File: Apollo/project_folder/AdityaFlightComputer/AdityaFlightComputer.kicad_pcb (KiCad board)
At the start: 2 copper layers, 52.3 x 83.4 mm, 18 parts, among them J1 SW, J2 BAT, J3 GPS, J4 Radio, U1 LPS22HHTR, U3 LSM6DSOTR, U4 MLX90397RLQ-AAA-000-SP

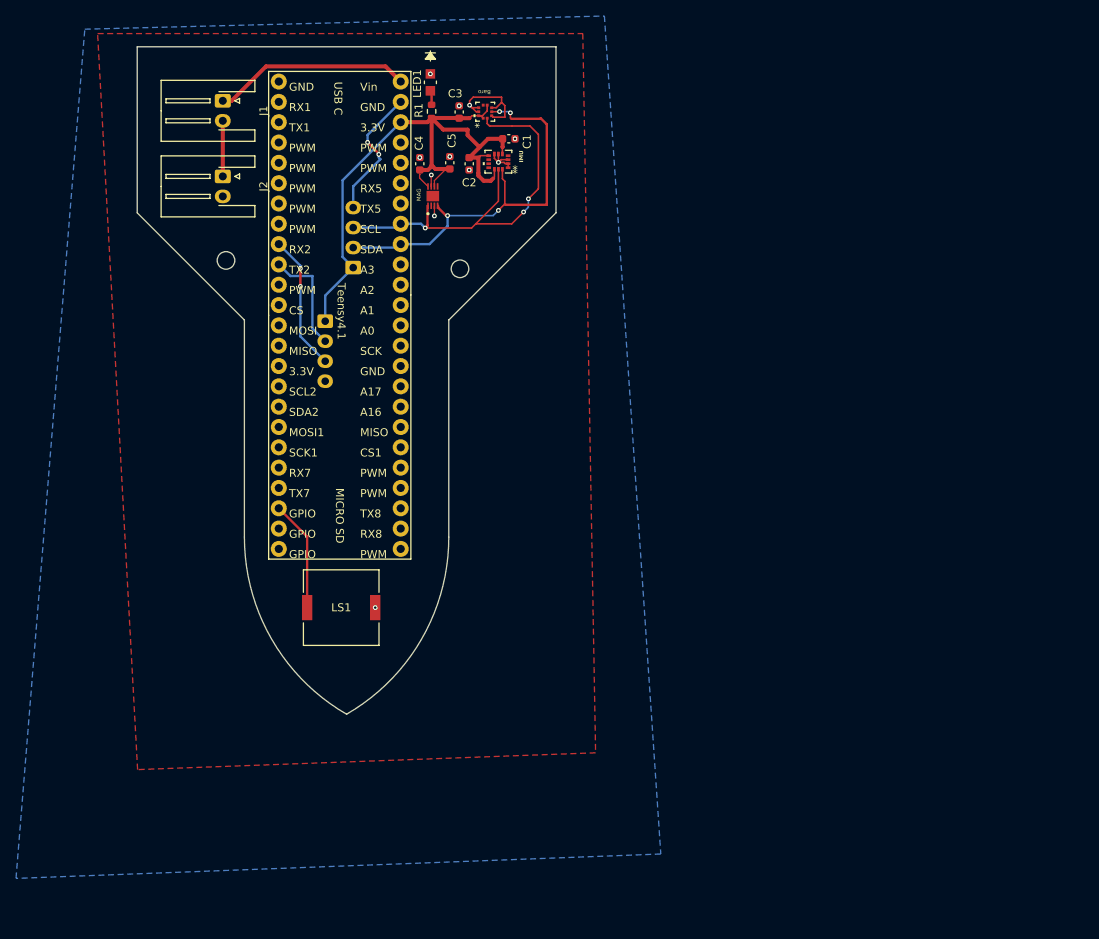
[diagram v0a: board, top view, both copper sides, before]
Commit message: autejwani
Fixed Flight Controller
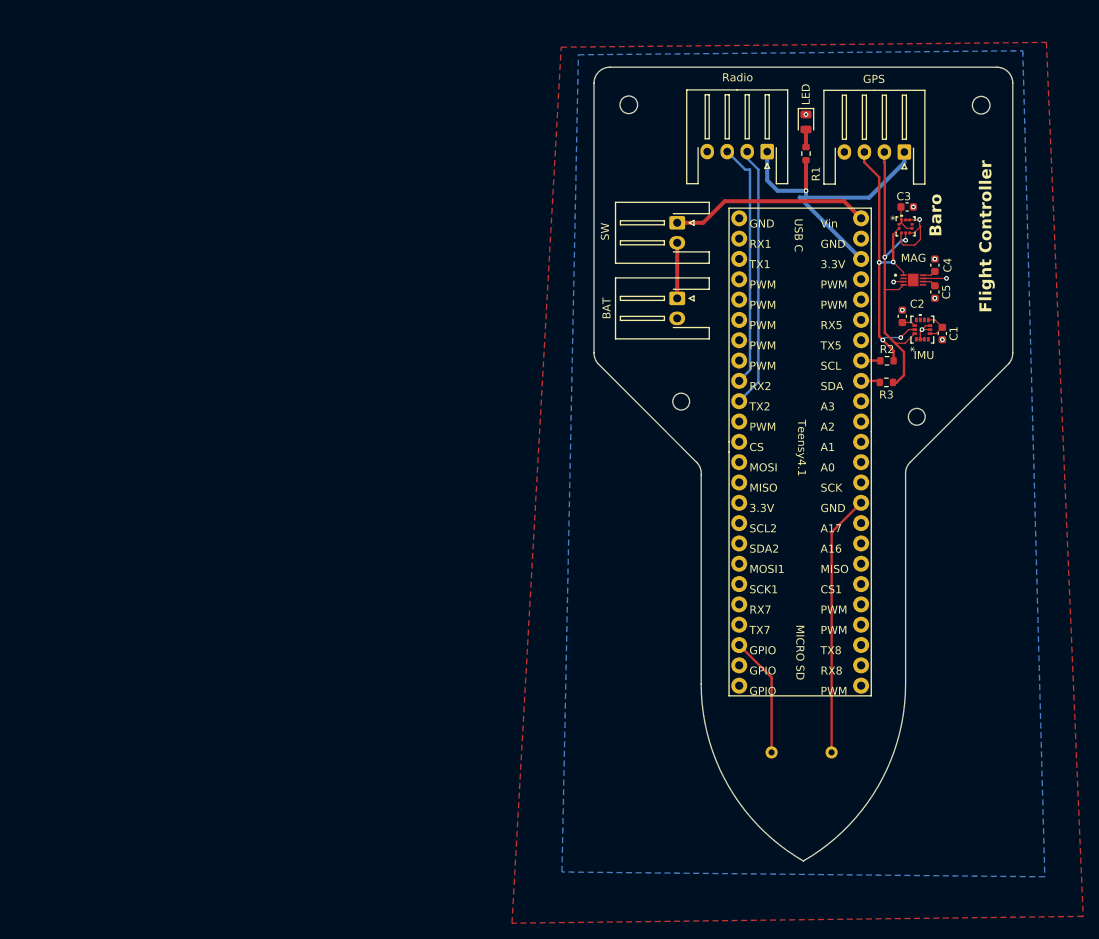
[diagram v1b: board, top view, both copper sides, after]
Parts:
- removed LED1: LTST-C170GKT, LTST-C170GKT:LED_LTST-C170GKT_LTO
- removed the REF** at (99.6, 55.2)
- removed the REF** at (128.8, 56.2)
- added D1: LED, LED_SMD:LED_0805_2012Metric, F.Cu at (172.1, 37.9)
- added R2: 5.1 k, Resistor_SMD:R_0603_1608Metric, F.Cu at (182.2, 67.8)
- added R3: 5.1 k, Resistor_SMD:R_0603_1608Metric, F.Cu at (182.2, 70.5)
- added REF**: MountingHole_2.2mm_M2, MountingHole:MountingHole_2.2mm_M2, F.Cu at (194.0, 35.8)
- added REF**: MountingHole_2.1mm, MountingHole:MountingHole_2.1mm, F.Cu at (156.5, 72.8)
- added REF**: MountingHole_2.1mm, MountingHole:MountingHole_2.1mm, F.Cu at (185.9, 74.8)
- added REF**: MountingHole_2.2mm_M2, MountingHole:MountingHole_2.2mm_M2, F.Cu at (149.9, 35.8)
- J3, J4: moved to F.Cu
- LS1: footprint CPT-9019A-SMT-TR:CPT-9019A_CUD -> CPT-9019A-SMT-TR:Adafruit_Buzzer; moved to B.Cu
- moved J3 70.4 mm to (184.4, 41.6), turned to 180 degrees
- moved C4 65.6 mm to (188.2, 55.8)
- moved C5 62.8 mm to (188.2, 59.1), turned to -90 degrees
- moved U4 61.0 mm to (185.5, 57.6), turned to 0 degrees
- moved LS1 60.6 mm to (171.8, 116.7)
- moved Teensy4.1 60.0 mm to (171.4, 79.2)
- moved C1 59.4 mm to (189.1, 64.3), turned to -90 degrees
- moved J4 59.2 mm to (167.2, 41.6), turned to 180 degrees
- moved J1 58.8 mm to (156.0, 50.5)
- moved J2 58.8 mm to (156.0, 60.0)
- moved C2 57.4 mm to (184.1, 62.2), turned to 90 degrees
- moved C3 57.2 mm to (184.7, 48.5), turned to 0 degrees
- moved U3 57.0 mm to (186.6, 63.9), turned to 90 degrees
- moved U1 54.5 mm to (184.6, 51.0), turned to 0 degrees
- moved R1 47.1 mm to (172.1, 41.9)
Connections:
- Teensy4.1 pad 18: SDA -> Net-(Teensy4.1-SDA)
- Teensy4.1 pad 19: SCL -> Net-(Teensy4.1-SCL)
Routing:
- net +3.3V: track 81.6 -> 54.0 mm, vias 0 -> 1
- net TX: track 13.6 -> 32.8 mm
- net RX: track 17.0 -> 30.8 mm, vias 2 -> 0
- net GND: track 38.5 -> 51.5 mm, vias 13 -> 10
- net SDA: track 51.6 -> 40.6 mm, vias 4 -> 2
- net SCL: track 51.5 -> 40.6 mm, vias 3 -> 4
- net Net-(Teensy4.1-SCL): track 0.00 -> 2.42 mm
- net Net-(Teensy4.1-SDA): track 0.00 -> 2.41 mm
- net Buzz_GPIO: track 13.9 -> 15.1 mm
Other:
- board size 52.3 x 83.4 mm -> 52.4 x 99.2 mm
- board text added: "Buzzer"
- board text added: "Flight Controller"
